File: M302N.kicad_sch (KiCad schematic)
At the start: 35 parts, among them J1 DC12V, J11 RJ45, J12 DC12V FAN, J13 Conn_01x05_Socket, J14 Conn_01x05_Socket, J15 Conn_01x05_Pin, J16 Conn_01x05_Pin, J17 Conn_01x08_Pin, J18 Conn_01x04_Socket, J19 Conn_01x04_Socket, J2 UART, J3 extend I/O, J4 I2C-1, J5 ADC_IN, J6 ADC_IN, J7 RESET, SW1 SW_Reed, U1 W5500, U2 NJM2845DL1-05

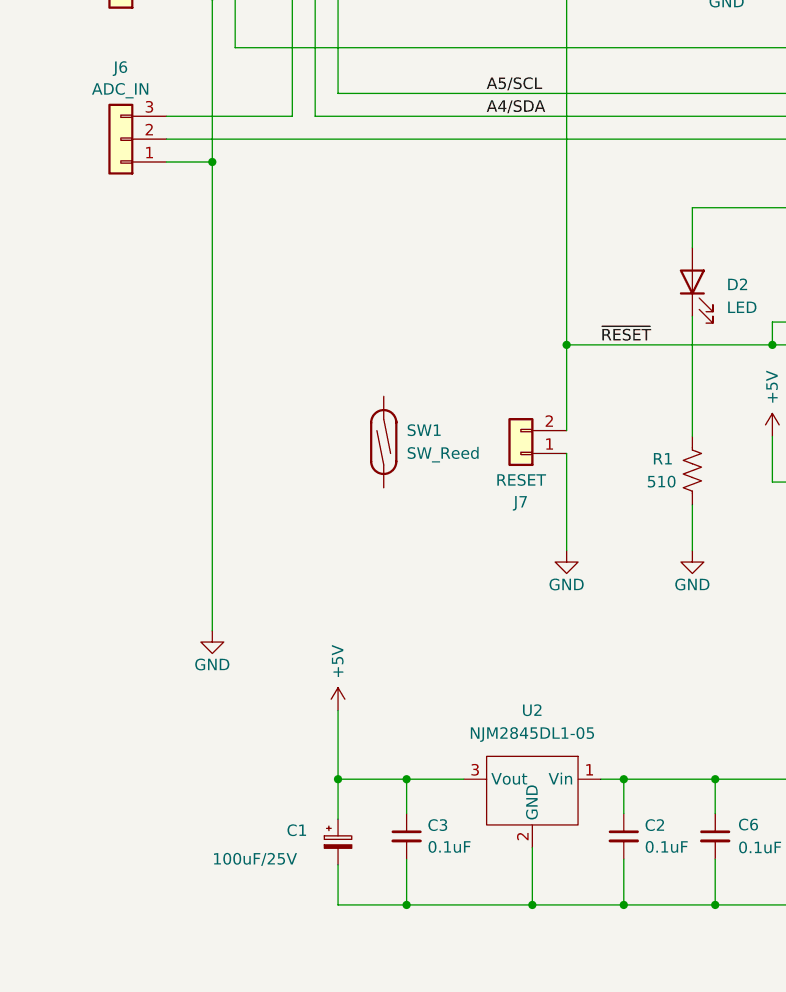
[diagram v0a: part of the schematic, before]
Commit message: DCDC converter
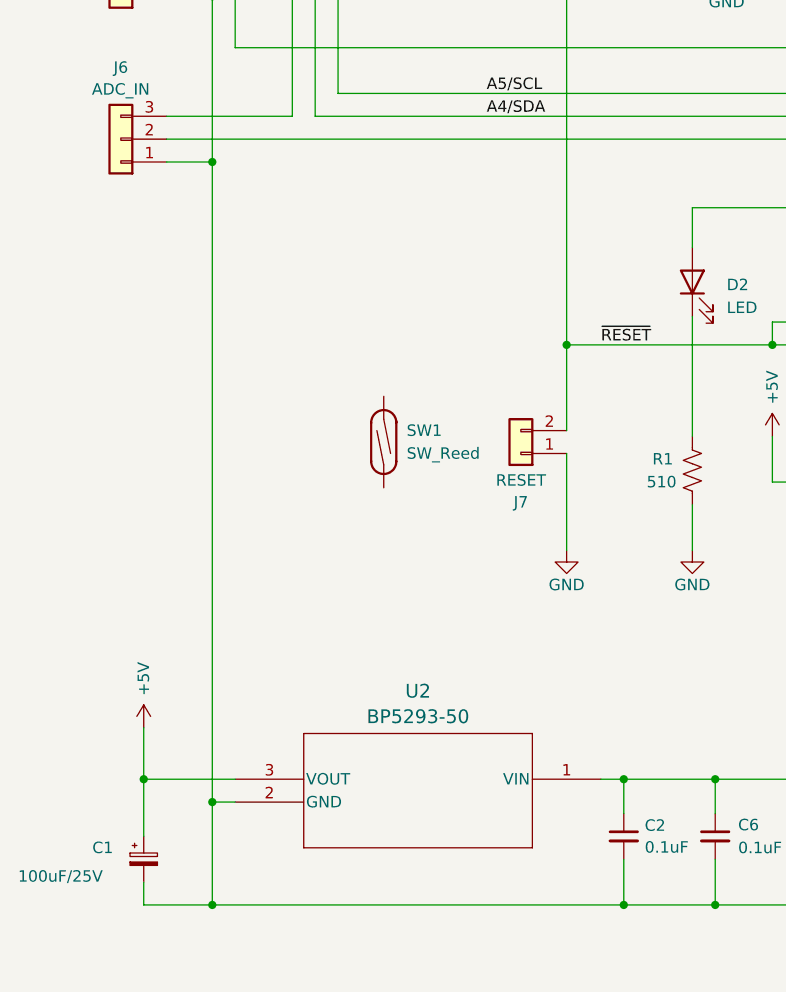
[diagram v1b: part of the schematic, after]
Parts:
- removed C3: 0.1uF, Capacitor_THT:C_Disc_D4.3mm_W1.9mm_P5.00mm, symbol Device:C_Small
- removed U2: NJM2845DL1-05, Package_TO_SOT_SMD:TO-252-3_TabPin2, symbol holly:NJM2845DL1
- added U2: BP5293-50, SIP03_BP5293_17X7P2_ROM, symbol 2025-06-02_10-47-13:BP5293-50
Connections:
- net +5V: now also U2.3 (VOUT)
- net GND: now also U2.2 (GND)
- net at C2.1, C5.1, C6.1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: now also U2.1 (VIN)
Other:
- moved on the sheet: C1
